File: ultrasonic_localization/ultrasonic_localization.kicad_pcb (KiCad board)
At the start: 2 copper layers, 69.6 x 80.4 mm, 212 parts, among them J101 USB_OTG_fix, J102 Conn_02x03_Odd_Even, J401 Screw_Terminal_1x02_Bat, Q101 BUK9Y29-40E, Q301 BC847, Q501 BC847, Q601 BC847, Q701 BC847, SW101 SW_Push, SW102 SW_DPDT, SW103 SW_DPDT, U101 ATMEGA32U4RC-AU, U102 MD0105, U103 4047, U201 nRF24L01+, U202 ANT016008LCS2442MA2, U301 LM324, U302 TCT40-16R/T, U401 AP3012, U402 AP3012, U403 TPS6223x, U404 LP5907SNX-3.3/NOPB, U405 BQ2423, U501 LM324, U502 TCT40-16R/T, U601 LM324, U602 TCT40-16R/T, U701 LM324, U702 TCT40-16R/T, U801 IMU, U802 Level_Shifter_4Channel, Y101 Crystal_GND24, Y201 16MHz

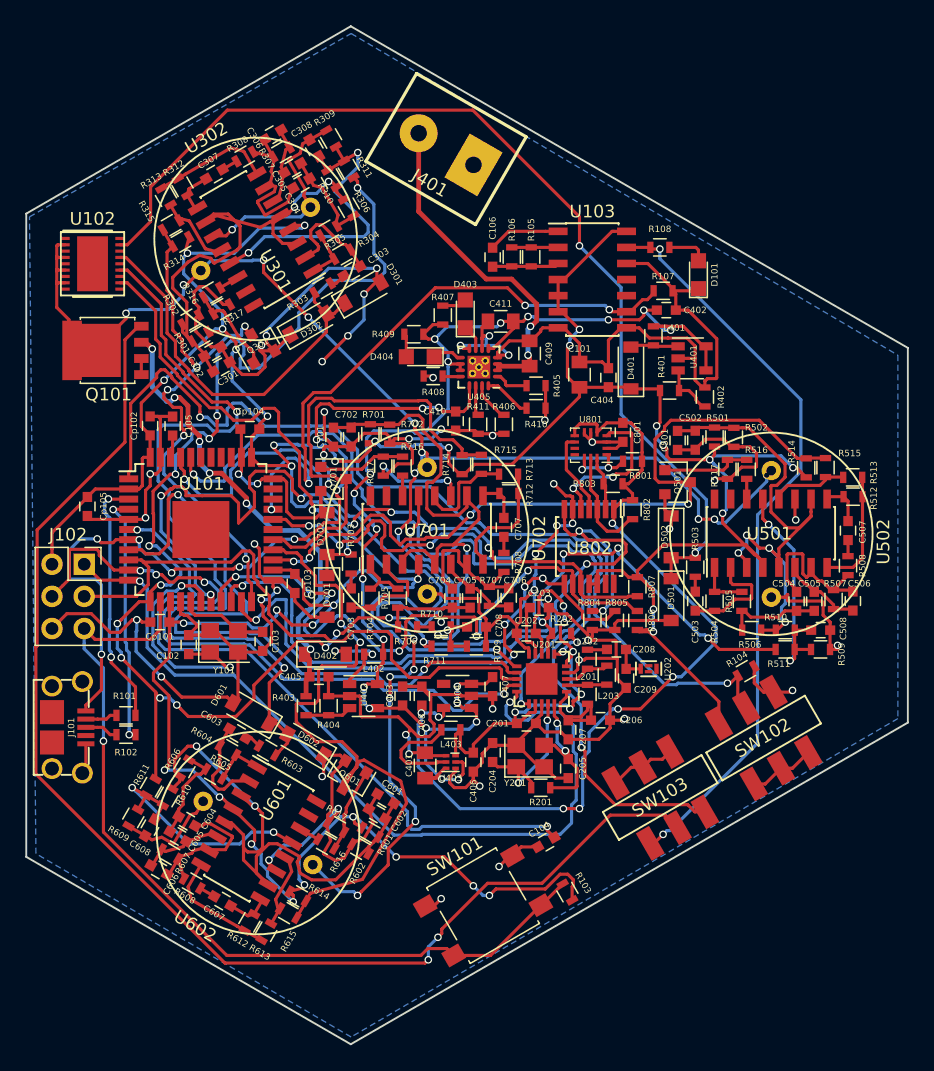
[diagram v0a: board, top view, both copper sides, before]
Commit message: finished routing with the new mux
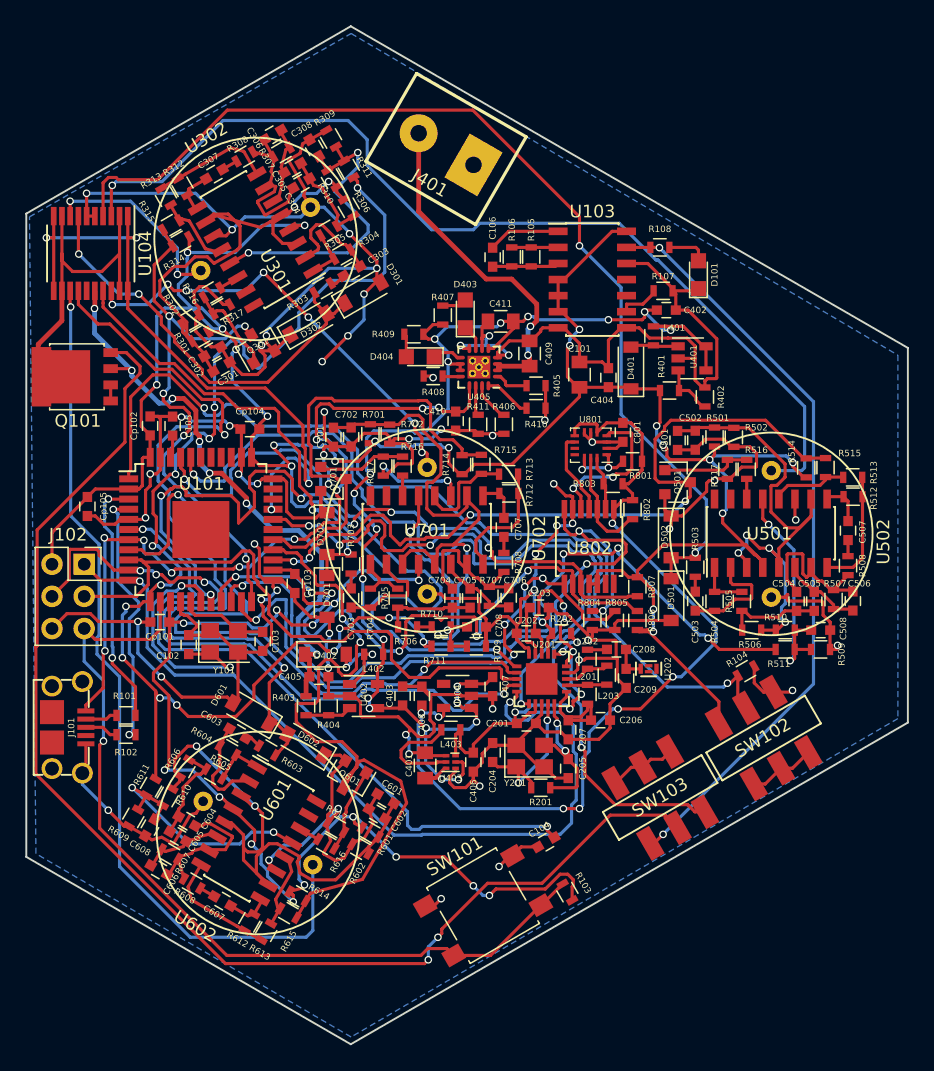
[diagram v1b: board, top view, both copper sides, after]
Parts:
- removed U102: MD0105, Custom:DFN-18-1EP_5x5mm_Pitch0.5mm
- added U104: ADG5434, Housings_SSOP:TSSOP-20_4.4x6.5mm_Pitch0.65mm, F.Cu at (74.9, 79.3)
- moved Q101 3.20 mm to (73.7, 89.1)
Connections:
- net /SW1b renamed /RX1
- net /SW2b renamed /RX2
- net /SW3b renamed /RX3
- net /SW4b renamed /RX4
- Q101 pad 5: /SW1a -> /TX
- R107 pad 1: /TX_EN -> Net-(R107-Pad1)
- U103 pad 9: /TX_EN -> Net-(R107-Pad1)
- U302 pad 1: /SW1a -> /UX2
- U502 pad 1: /SW1a -> /UX1
- U602 pad 1: /SW1a -> /UX3
- U702 pad 1: /SW1a -> /UX4
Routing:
- net /SW1a: track 138.4 -> 0.00 mm, vias 17 -> 0
- net /UX1: track 0.00 -> 78.3 mm, vias 0 -> 1
- net /UX3: track 0.00 -> 70.2 mm, vias 0 -> 1
- net GND: track 446.0 -> 486.0 mm, vias 54 -> 58
- net /UX4: track 0.00 -> 35.5 mm, vias 0 -> 7
- net /TX: track 0.00 -> 25.7 mm
- net /UX2: track 0.00 -> 15.2 mm, vias 0 -> 2
- net /+26V: track 38.5 -> 47.4 mm, vias 6 -> 7
- net +5V: track 297.4 -> 302.3 mm
- net /TX_EN: track 47.3 -> 51.8 mm
- net /USB5V: track 65.6 -> 61.4 mm
- net /RX2: track 30.4 -> 34.1 mm, vias 0 -> 2
- net Net-(R107-Pad1): track 0.00 -> 3.29 mm
- net /ID: track 76.6 -> 74.8 mm
- net /SIG3: track 53.2 -> 54.6 mm
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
